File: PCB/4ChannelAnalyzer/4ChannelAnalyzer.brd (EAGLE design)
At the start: 64.8 x 91.4 mm, 21 parts, among them U1-ADD-49 ADS1015IDGST, U2-ADD-48 ADS1015IDGST, U3 LM1117MP-3.3, X3 MINI-USB-32005-301

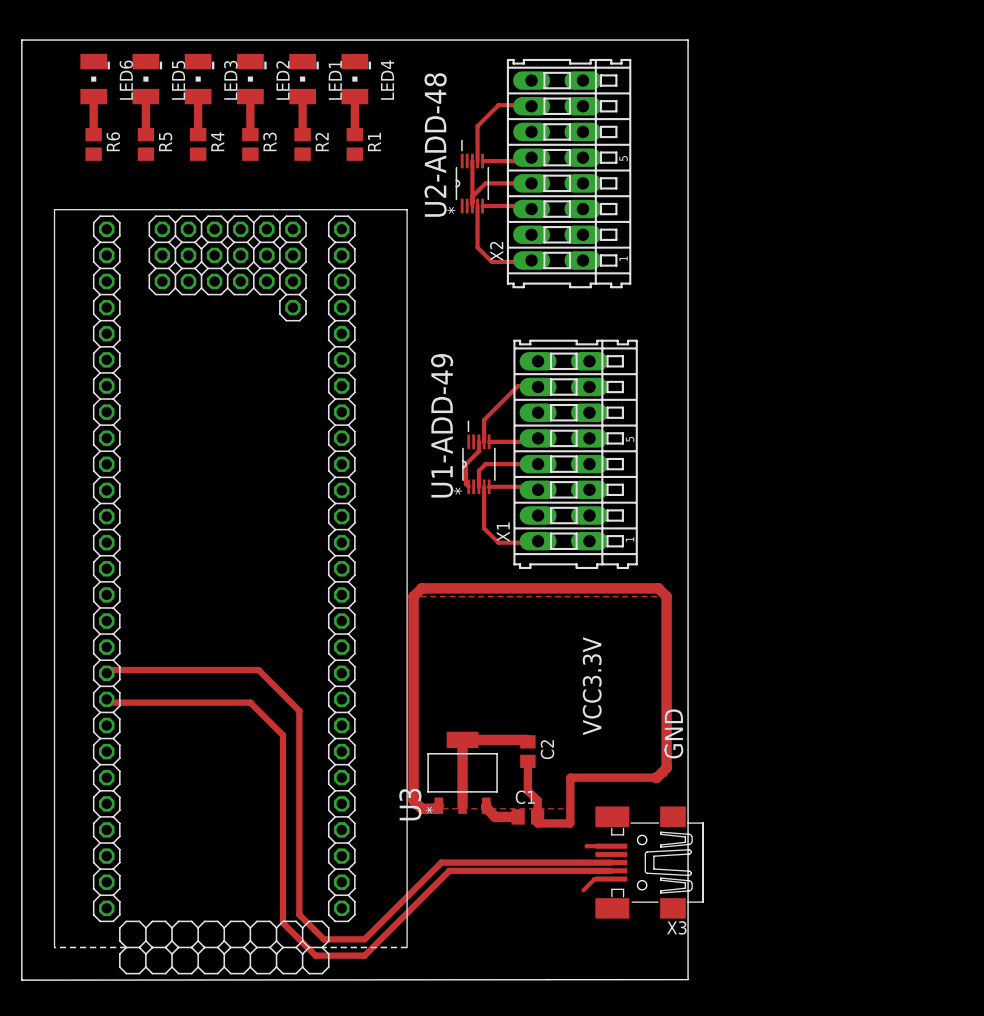
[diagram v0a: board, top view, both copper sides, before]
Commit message: Wiring sensors connectors.
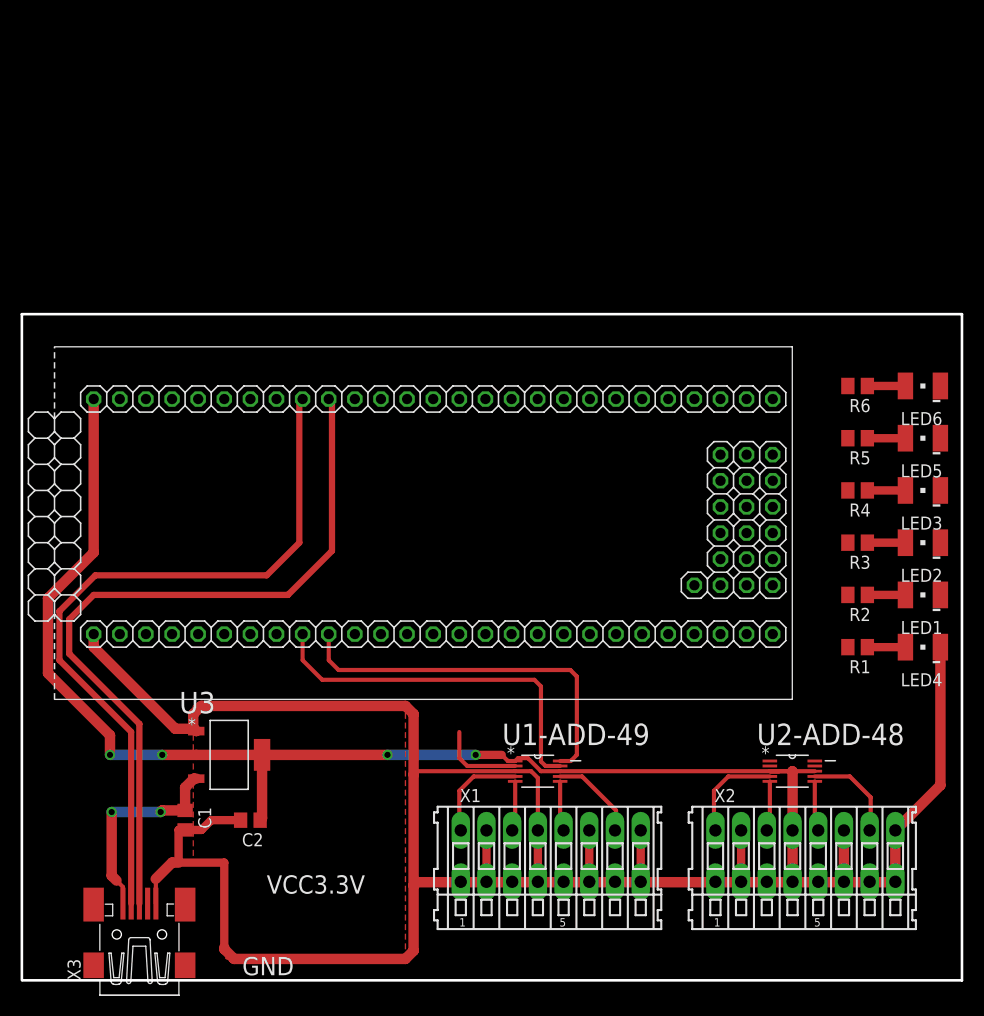
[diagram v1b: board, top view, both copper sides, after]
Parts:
- moved LED6 86.0 mm to (87.6, 57.8), turned to 90 degrees
- moved LED5 83.2 mm to (87.6, 52.7), turned to 90 degrees
- moved LED3 81.0 mm to (87.6, 47.6), turned to 90 degrees
- moved LED2 79.4 mm to (87.6, 42.5), turned to 90 degrees
- moved LED1 78.5 mm to (87.6, 37.5), turned to 90 degrees
- moved LED4 78.1 mm to (87.6, 32.4), turned to 90 degrees
- moved R6 77.9 mm to (81.3, 57.8), turned to 180 degrees
- moved R5 74.9 mm to (81.3, 52.7), turned to 180 degrees
- moved R4 72.4 mm to (81.3, 47.6), turned to 180 degrees
- moved X2 70.9 mm to (76.2, 12.1), turned to 0 degrees
- moved R3 70.6 mm to (81.3, 42.5), turned to 180 degrees
- moved R2 69.5 mm to (81.3, 37.5), turned to 180 degrees
- moved R1 69.1 mm to (81.3, 32.4), turned to 180 degrees
- moved U2-ADD-48 65.1 mm to (74.9, 20.3), turned to 0 degrees
- moved X3 49.4 mm to (11.4, 4.45), turned to 90 degrees
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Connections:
- net GND: now also LPC1.1
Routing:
- net GND: track 105.7 -> 243.2 mm
- net VCC3.3V: track 21.9 -> 114.8 mm, vias 0 -> 4
- net SCL49: track 0.00 -> 36.8 mm
- net SDA49: track 0.00 -> 36.1 mm
- net USB-5V: track 6.85 -> 20.3 mm, vias 0 -> 2
- net EXT_INT_0: track 0.00 -> 8.29 mm
- net N$19: track 73.5 -> 71.5 mm
- net N$20: track 74.8 -> 73.7 mm
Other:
- board size 64.8 x 91.4 mm -> 91.4 x 64.8 mm
- board text added: "Sensors Connectors"
